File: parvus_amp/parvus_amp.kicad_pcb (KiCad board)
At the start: 2 copper layers, 70 x 54 mm, 45 parts, among them J1 ctrl, J2 input, J3 output, J4 power, U1 TDA7293

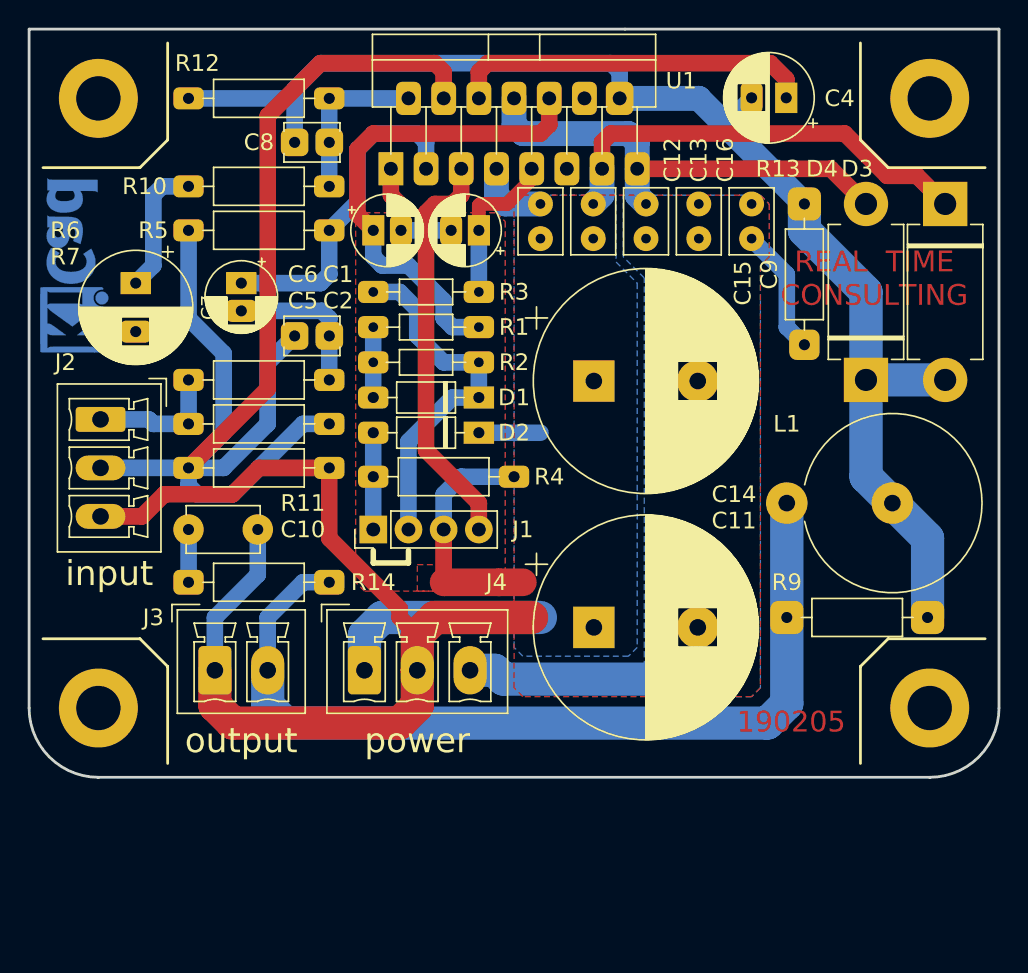
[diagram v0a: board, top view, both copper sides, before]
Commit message: Prerelease of version 1.02
Signed-off-by: Nenad Radulovic <nenad.b.radulovic@gmail.com>
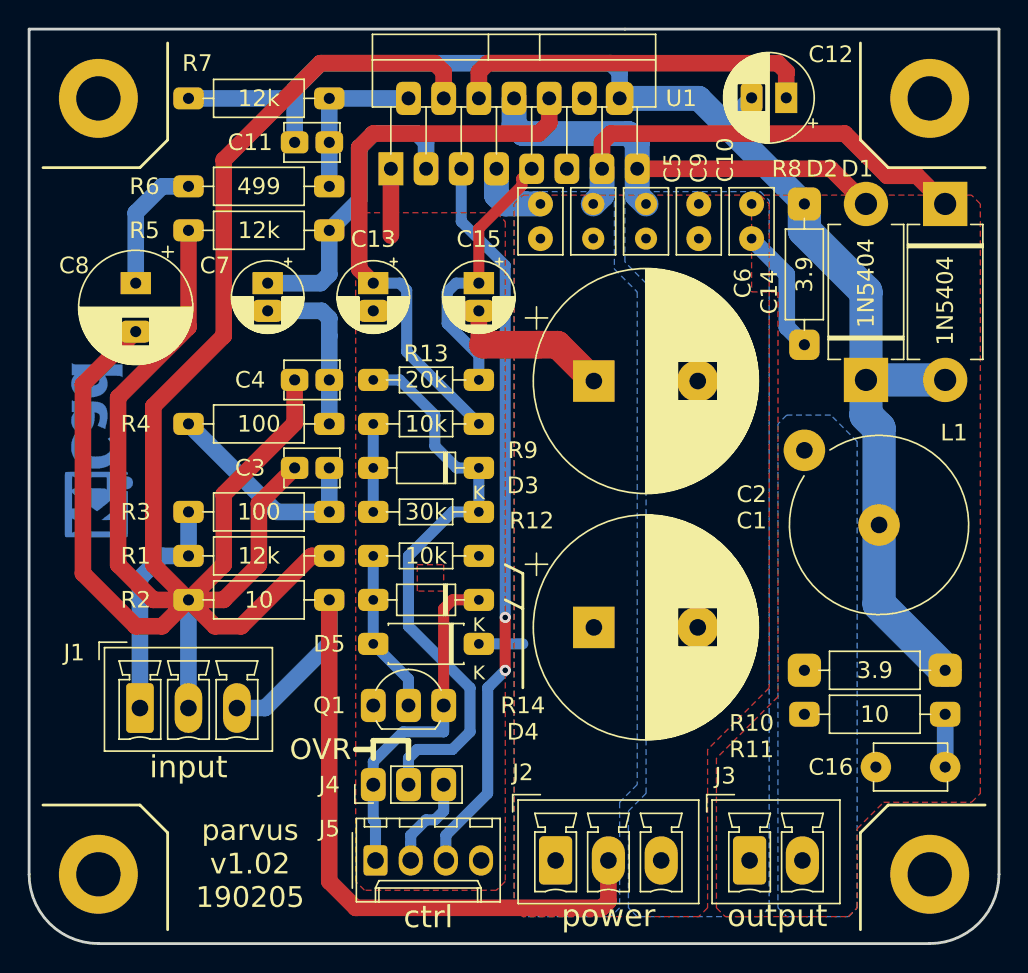
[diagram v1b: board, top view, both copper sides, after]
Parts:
- removed the C11 at (128.3, 91.6)
- removed the C7 at (95.2, 66.8)
- removed the D1 at (120.0, 75.0)
- removed the D2 at (120.0, 77.5)
- removed the J1 at (112.3, 84.5)
- removed the R1 at (112.3, 69.9)
- removed the R10 at (109.2, 59.8)
- removed the R2 at (120.0, 72.5)
- removed the R4 at (122.5, 80.7)
- added C13: 10u, Capacitor_THT:CP_Radial_D5.0mm_P2.00mm, F.Cu at (112.3, 66.8)
- added C3: 220p, Capacitor_THT:C_Disc_D3.8mm_W2.6mm_P2.50mm, F.Cu at (109.2, 80.1)
- added C8: 470u, Capacitor_THT:CP_Radial_D8.0mm_P3.50mm, F.Cu at (95.2, 66.8)
- added D3: 1N4148, Diode_THT:D_DO-35_SOD27_P7.62mm_Horizontal, F.Cu at (120.0, 80.1)
- added D4: 1N4148, Diode_THT:D_DO-35_SOD27_P7.62mm_Horizontal, F.Cu at (120.0, 89.6)
- added D5: 1N5246B, Diode_THT:D_DO-41_SOD81_P7.62mm_Horizontal, F.Cu at (120.0, 92.8)
- added J4: ctrl_override, Connector_PinHeader_2.54mm:PinHeader_1x03_P2.54mm_Vertical, F.Cu at (112.3, 103.0)
- added J5: ctrl, Connector_Molex:Molex_KK-254_AE-6410-04A_1x04_P2.54mm_Vertical, F.Cu at (112.5, 108.4)
- added Q1: BC556B, Package_TO_SOT_THT:TO-92L_Inline_Wide, F.Cu at (112.3, 97.2)
- added R11: 10, Resistor_THT:R_Axial_DIN0207_L6.3mm_D2.5mm_P10.16mm_Horizontal, F.Cu at (143.5, 97.9)
- added R12: 30k, Resistor_THT:R_Axial_DIN0204_L3.6mm_D1.6mm_P7.62mm_Horizontal, F.Cu at (120.0, 83.3)
- added R3: 100, Resistor_THT:R_Axial_DIN0207_L6.3mm_D2.5mm_P10.16mm_Horizontal, F.Cu at (109.2, 83.3)
- added R6: 499, Resistor_THT:R_Axial_DIN0207_L6.3mm_D2.5mm_P10.16mm_Horizontal, F.Cu at (109.2, 59.8)
- added R9: 10k, Resistor_THT:R_Axial_DIN0204_L3.6mm_D1.6mm_P7.62mm_Horizontal, F.Cu at (112.3, 76.9)
- C1: value 10u -> 2m2; footprint Capacitor_THT:CP_Radial_D5.0mm_P2.00mm -> Capacitor_THT:CP_Radial_D16.0mm_P7.50mm
- C7: renamed from C6; value 3u3 -> 22u
- R13: renamed from R3; value 30k -> 20k
- R14: value 10 -> 10k; footprint Resistor_THT:R_Axial_DIN0207_L6.3mm_D2.5mm_P10.16mm_Horizontal -> Resistor_THT:R_Axial_DIN0204_L3.6mm_D1.6mm_P7.62mm_Horizontal
- moved C16 57.2 mm to (153.6, 101.7), turned to 180 degrees
- moved J3 41.0 mm to (139.5, 108.4)
- moved C1 32.8 mm to (128.3, 91.6)
- moved J1 21.0 mm to (95.5, 97.4), turned to 0 degrees
- moved J2 19.5 mm to (125.5, 108.4)
- moved NT1 17.4 mm to (122.2, 71.2)
- moved LOGO1 13.5 mm to (92.0, 78.8)
- moved MK1 12.0 mm to (92.5, 109.4)
- moved MK4 12.0 mm to (152.5, 109.4)
- moved R14 11.0 mm to (120.0, 86.4)
- moved R1 9.52 mm to (109.2, 86.4)
- moved R2 9.52 mm to (99.0, 89.6)
- moved R13 6.35 mm to (112.3, 73.7)
- moved R10 4.02 mm to (143.5, 94.7)
- moved C15 3.81 mm to (120.0, 66.8), turned to 270 degrees
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- renumbered C16 to C10, C8 to C11, C4 to C12, C9 to C14, C2 to C15, C10 to C16, C14 to C2, C5 to C4, C12 to C5, C15 to C6, C13 to C9, D3 to D1, D4 to D2, J2 to J1, J4 to J2, MK3 to MK2, MK2 to MK3, R7 to R1, R9 to R10, R11 to R2, R6 to R4, R12 to R7, R13 to R8
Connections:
- C1 pad 1: /mute -> +pwvs
- C1 pad 2: GNDD -> GNDPWR
- C16 pad 1: Net-(C10-Pad1) -> Net-(C16-Pad1)
- R14 pad 1: /out -> GNDD
- R14 pad 2: Net-(C10-Pad1) -> Net-(D4-Pad2)
- R4 pad 2: /input -> Net-(C3-Pad1)
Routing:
- net /sgnd: track 102.0 -> 171.3 mm
- net /out: track 64.9 -> 0.00 mm
- net Net-(D4-Pad1): track 0.00 -> 24.9 mm
- net Net-(J5-Pad3): track 29.4 -> 53.0 mm, vias 0 -> 2
- net +pwvs: track 57.3 -> 40.3 mm
- net Net-(D3-Pad1): track 26.1 -> 42.8 mm
- net GNDPWR: track 77.9 -> 61.3 mm
- net Net-(C3-Pad1): track 0.00 -> 16.0 mm
- net -pwvs: track 48.2 -> 33.6 mm
- net GNDD: track 20.3 -> 7.39 mm
- net Net-(D4-Pad2): track 0.00 -> 11.8 mm
- net Net-(C8-Pad1): track 0.00 -> 9.68 mm
- net Net-(C7-Pad1) (its old number): track 9.68 -> 0.00 mm
- net /stby: track 11.6 -> 19.7 mm
- net /input: track 9.66 -> 16.7 mm
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- added copper zone on B.Cu, net /out
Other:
- board size 70 x 54 mm -> 70 x 66 mm
- board text added: "+/PG out"
- board text added: "56mm"
- board text added: "DG/C/O/VS"
- board text added: "OVR"
- board text added: "parvus v1.02 190205"
- board text removed: "190205"
- board text removed: "44mm"
- board text removed: "PG/+ out"
- board text removed: "parvus v1.01"
